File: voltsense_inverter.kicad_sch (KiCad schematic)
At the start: 9 parts, among them J17 Capacitor connector, U3 Opamp_Quad

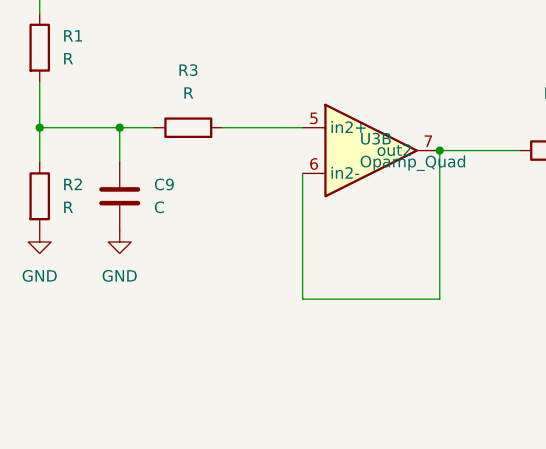
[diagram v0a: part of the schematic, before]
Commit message: Autosave
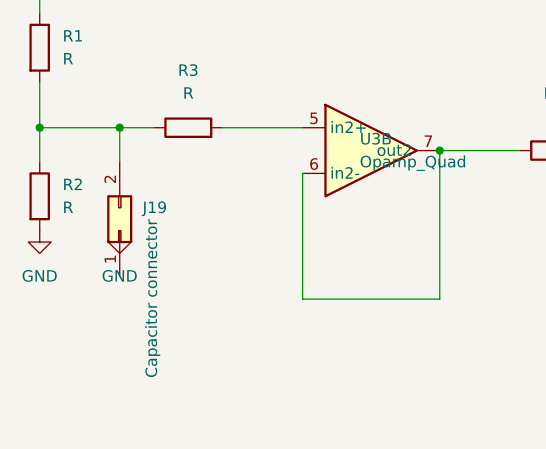
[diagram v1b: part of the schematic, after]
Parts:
- removed C9: C, symbol Device:C
- added J19: Capacitor connector, symbol Connector_Generic:Conn_02x01
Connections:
- net at R1.2, R2.1, R3.1: now also J19.2 (Pin_2)
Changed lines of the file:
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@@
+	)
+	(symbol
+		(lib_id "Connector_Generic:Conn_02x01")
+		(at 62.23 59.69 90)
+		(unit 1)
+		(body_style 1)
+		(exclude_from_sim no)
+		(in_bom yes)
+		(on_board yes)
+		(in_pos_files yes)
+		(dnp no)
+		(property "Reference" "J19"
+			(at 64.77 57.1499 90)
+			(show_name no)
+			(do_not_autoplace no)
+			(effects
+				(font
+					(size 1.27 1.27)
+				)
+				(justify right)
+			)
+		)
+		(property "Value" "Capacitor connector"
+			(at 65.786 58.42 0)
+			(show_name no)
+			(do_not_autoplace no)
+			(effects
+				(font
+					(size 1.27 1.27)
+				)
+				(justify right)
+			)
+		)
+		(property "Footprint" ""
+			(at 62.23 59.69 0)
+			(hide yes)
+			(show_name no)
+			(do_not_autoplace no)
+			(effects
+				(font
+					(size 1.27 1.27)
+				)
+			)
+		)
+		(property "Datasheet" ""
+			(at 62.23 59.69 0)
+			(hide yes)
+			(show_name no)
+			(do_not_autoplace no)
+			(effects
+				(font
+					(size 1.27 1.27)
+				)
+			)
+		)
+		(property "Description" "Generic connector, double row, 02x01, this symbol is compatible with counter-clockwise, top-bottom and odd-even numbering schemes., script generated (kicad-library-utils/schlib/autogen/connector/)"
+			(at 62.23 59.69 0)
+			(hide yes)
+			(show_name no)
+			(do_not_autoplace no)
+			(effects
+				(font
+					(size 1.27 1.27)
+				)
+			)
+		)
+		(pin "2"
+		)
+		(pin "1"
+		)
+		(instances
+			(project "WET_PCB_v2"
+				(path "/13451c35-1666-47d9-9525-8d8125ba1cf3/419c9796-b7e1-43c1-b033-dc2479750a67"
+					(reference "J19")
+					(unit 1)
+				)
+			)
+		)
 	)
 	(symbol
@@
 				)
 			)
-		)
-	)
-	(symbol
-		(lib_id "Device:C")
-		(at 62.23 55.88 0)
-		(unit 1)
-		(body_style 1)
-		(exclude_from_sim no)
-		(in_bom yes)
-		(on_board yes)
-		(in_pos_files yes)
-		(dnp no)
-		(fields_autoplaced yes)
-		(property "Reference" "C9"
-			(at 66.04 54.6099 0)
-			(show_name no)
-			(do_not_autoplace no)
-			(effects
-				(font
-					(size 1.27 1.27)
-				)
-				(justify left)
-			)
-		)
-		(property "Value" "C"
-			(at 66.04 57.1499 0)
-			(show_name no)
-			(do_not_autoplace no)
-			(effects
-				(font
-					(size 1.27 1.27)
-				)
-				(justify left)
-			)
-		)
-		(property "Footprint" ""
-			(at 63.1952 59.69 0)
-			(hide yes)
-			(show_name no)
-			(do_not_autoplace no)
-			(effects
-				(font
-					(size 1.27 1.27)
-				)
-			)
-		)
-		(property "Datasheet" ""
-			(at 62.23 55.88 0)
-			(hide yes)
-			(show_name no)
-			(do_not_autoplace no)
-			(effects
-				(font
-					(size 1.27 1.27)
-				)
-			)
-		)
-		(property "Description" "Unpolarized capacitor"
-			(at 62.23 55.88 0)
-			(hide yes)
-			(show_name no)
-			(do_not_autoplace no)
-			(effects
-				(font
-					(size 1.27 1.27)
-				)
-			)
-		)
-		(pin "1"
-		)
-		(pin "2"
-		)
-		(instances
-			(project "WET_PCB_v2"
-				(path "/13451c35-1666-47d9-9525-8d8125ba1cf3/419c9796-b7e1-43c1-b033-dc2479750a67"
-					(reference "C9")
-					(unit 1)
-				)
-			)

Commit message: SCH Save: 2 files changed voltsense_inverter.kicad_sch 156/0/81 WET_PCB_v2.kicad_pro 0/0/1
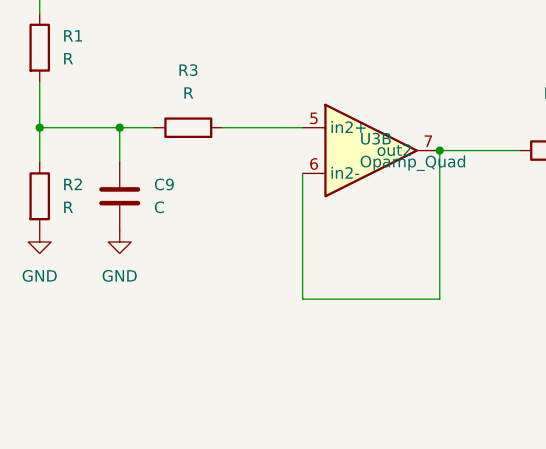
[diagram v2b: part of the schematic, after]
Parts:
- removed J19: Capacitor connector, symbol Connector_Generic:Conn_02x01
- added C9: C, symbol Device:C
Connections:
- net GND: now also C9.2
- net at R1.2, R2.1, R3.1: now also C9.1
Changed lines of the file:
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@@
-	)
-	(symbol
-		(lib_id "Connector_Generic:Conn_02x01")
-		(at 62.23 59.69 90)
-		(unit 1)
-		(body_style 1)
-		(exclude_from_sim no)
-		(in_bom yes)
-		(on_board yes)
-		(in_pos_files yes)
-		(dnp no)
-		(property "Reference" "J19"
-			(at 64.77 57.1499 90)
-			(show_name no)
-			(do_not_autoplace no)
-			(effects
-				(font
-					(size 1.27 1.27)
-				)
-				(justify right)
-			)
-		)
-		(property "Value" "Capacitor connector"
-			(at 65.786 58.42 0)
-			(show_name no)
-			(do_not_autoplace no)
-			(effects
-				(font
-					(size 1.27 1.27)
-				)
-				(justify right)
-			)
-		)
-		(property "Footprint" ""
-			(at 62.23 59.69 0)
-			(hide yes)
-			(show_name no)
-			(do_not_autoplace no)
-			(effects
-				(font
-					(size 1.27 1.27)
-				)
-			)
-		)
-		(property "Datasheet" ""
-			(at 62.23 59.69 0)
-			(hide yes)
-			(show_name no)
-			(do_not_autoplace no)
-			(effects
-				(font
-					(size 1.27 1.27)
-				)
-			)
-		)
-		(property "Description" "Generic connector, double row, 02x01, this symbol is compatible with counter-clockwise, top-bottom and odd-even numbering schemes., script generated (kicad-library-utils/schlib/autogen/connector/)"
-			(at 62.23 59.69 0)
-			(hide yes)
-			(show_name no)
-			(do_not_autoplace no)
-			(effects
-				(font
-					(size 1.27 1.27)
-				)
-			)
-		)
-		(pin "2"
-		)
-		(pin "1"
-		)
-		(instances
-			(project "WET_PCB_v2"
-				(path "/13451c35-1666-47d9-9525-8d8125ba1cf3/419c9796-b7e1-43c1-b033-dc2479750a67"
-					(reference "J19")
-					(unit 1)
-				)
-			)
-		)
 	)
 	(symbol
@@
 				)
 			)
+		)
+	)
+	(symbol
+		(lib_id "Device:C")
+		(at 62.23 55.88 0)
+		(unit 1)
+		(body_style 1)
+		(exclude_from_sim no)
+		(in_bom yes)
+		(on_board yes)
+		(in_pos_files yes)
+		(dnp no)
+		(fields_autoplaced yes)
+		(property "Reference" "C9"
+			(at 66.04 54.6099 0)
+			(show_name no)
+			(do_not_autoplace no)
+			(effects
+				(font
+					(size 1.27 1.27)
+				)
+				(justify left)
+			)
+		)
+		(property "Value" "C"
+			(at 66.04 57.1499 0)
+			(show_name no)
+			(do_not_autoplace no)
+			(effects
+				(font
+					(size 1.27 1.27)
+				)
+				(justify left)
+			)
+		)
+		(property "Footprint" ""
+			(at 63.1952 59.69 0)
+			(hide yes)
+			(show_name no)
+			(do_not_autoplace no)
+			(effects
+				(font
+					(size 1.27 1.27)
+				)
+			)
+		)
+		(property "Datasheet" ""
+			(at 62.23 55.88 0)
+			(hide yes)
+			(show_name no)
+			(do_not_autoplace no)
+			(effects
+				(font
+					(size 1.27 1.27)
+				)
+			)
+		)
+		(property "Description" "Unpolarized capacitor"
+			(at 62.23 55.88 0)
+			(hide yes)
+			(show_name no)
+			(do_not_autoplace no)
+			(effects
+				(font
+					(size 1.27 1.27)
+				)
+			)
+		)
+		(pin "1"
+		)
+		(pin "2"
+		)
+		(instances
+			(project "WET_PCB_v2"
+				(path "/13451c35-1666-47d9-9525-8d8125ba1cf3/419c9796-b7e1-43c1-b033-dc2479750a67"
+					(reference "C9")
+					(unit 1)
+				)
+			)

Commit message: SCH Save: 4 files changed currsense_DCDC.kicad_sch 0/0/4 decoration.kicad_sch 0/0/12 voltsense_DCDC.kicad_sch 0/0/4 voltsense_inverter.kicad_sch 0/0/4
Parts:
- R1, R2, R3, R4: footprint Resistor_THT:R_Axial_DIN0207_L6.3mm_D2.5mm_P7.62mm_Horizontal -> (none)
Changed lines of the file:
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@@
 			)
 		)
-		(property "Footprint" "Resistor_THT:R_Axial_DIN0207_L6.3mm_D2.5mm_P7.62mm_Horizontal"
+		(property "Footprint" ""
 			(at 110.49 52.578 90)
 			(hide yes)
@@
 			)
 		)
-		(property "Footprint" "Resistor_THT:R_Axial_DIN0207_L6.3mm_D2.5mm_P7.62mm_Horizontal"
+		(property "Footprint" ""
 			(at 51.562 55.88 90)
 			(hide yes)
@@
 			)
 		)
-		(property "Footprint" "Resistor_THT:R_Axial_DIN0207_L6.3mm_D2.5mm_P7.62mm_Horizontal"
+		(property "Footprint" ""
 			(at 69.85 50.038 90)
 			(hide yes)
@@
 			)
 		)
-		(property "Footprint" "Resistor_THT:R_Axial_DIN0207_L6.3mm_D2.5mm_P7.62mm_Horizontal"
+		(property "Footprint" ""
 			(at 51.562 39.37 90)
 			(hide yes)
